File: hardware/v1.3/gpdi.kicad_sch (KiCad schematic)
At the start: 19 parts, among them J2 GPDI_C_1.3, U1 ECP5-CABGA256, U5 PCA9306DC1

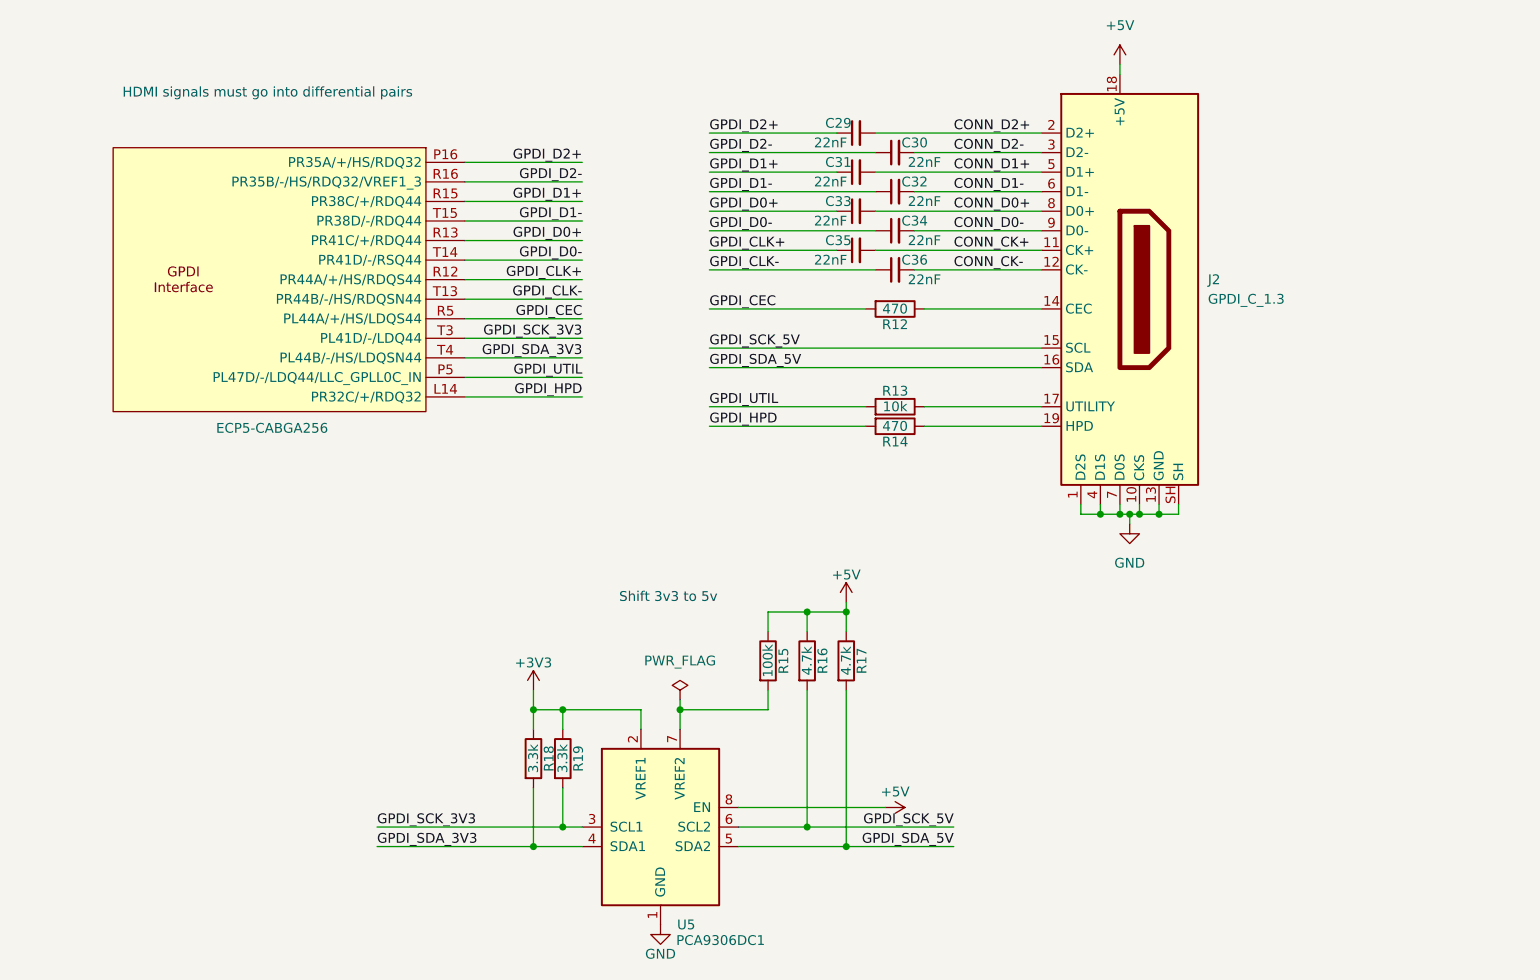
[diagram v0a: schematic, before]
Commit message: Update files
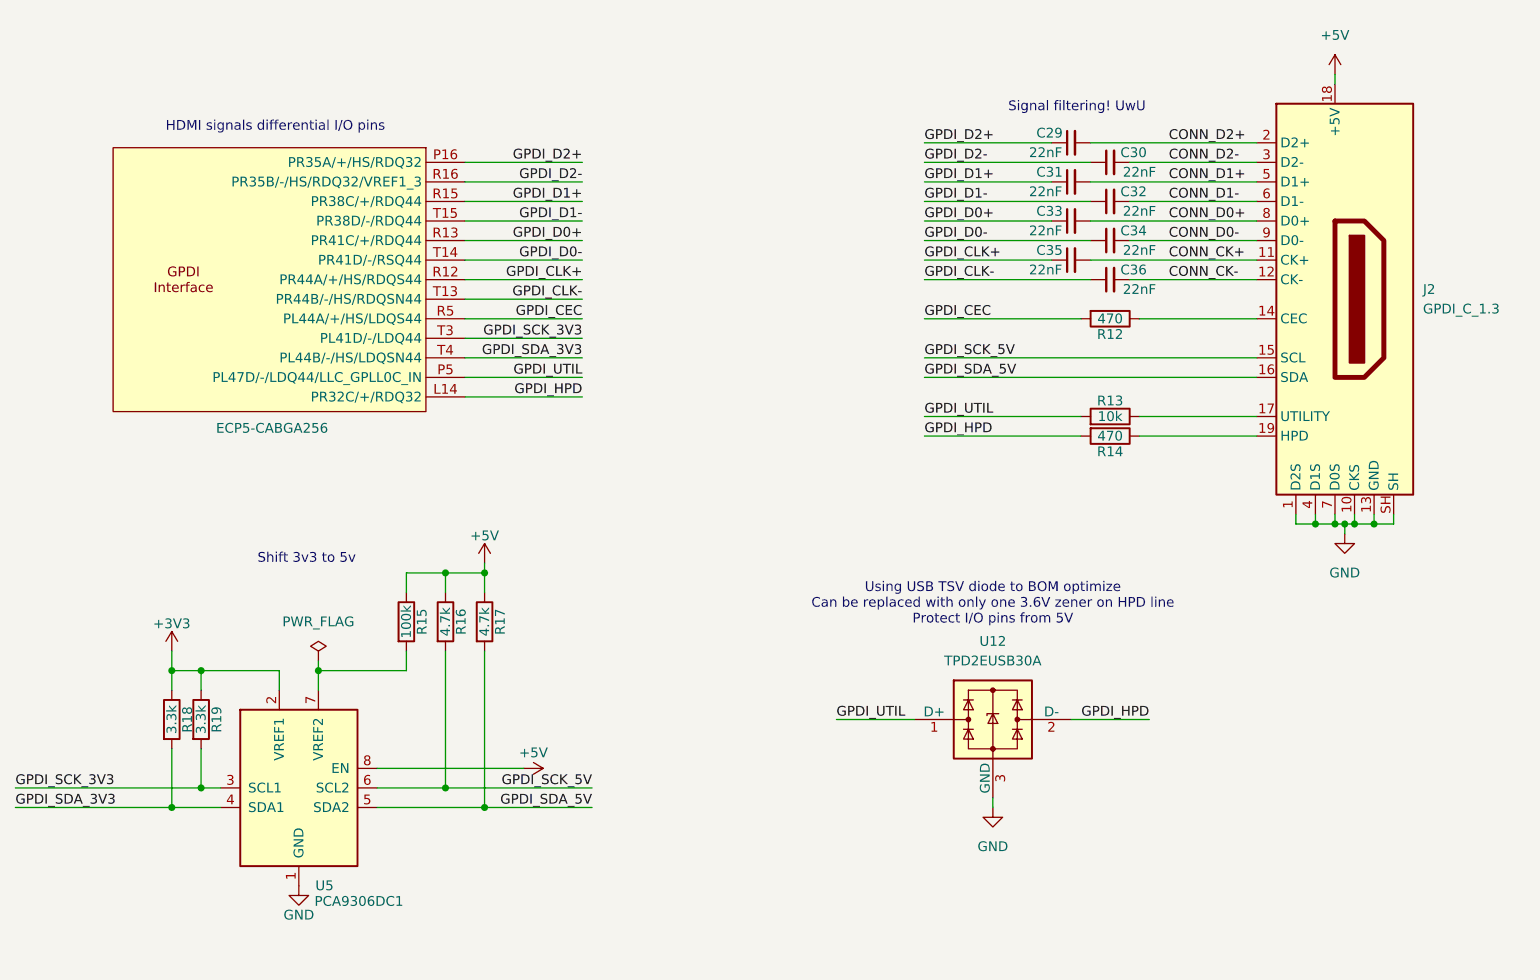
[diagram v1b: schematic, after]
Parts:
- added U12: TPD2EUSB30A, Package_TO_SOT_SMD:Texas_DRT-3, symbol Power_Protection:TPD2EUSB30A
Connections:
- net GND: now also U12.3 (GND)
- net GPDI_HPD: now also U12.2 (D-)
- net GPDI_UTIL: now also U12.1 (D+)
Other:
- note added: "HDMI signals differential I/O pins"
- note added: "Signal filtering! UwU"
- note added: "Using USB TSV diode to BOM optimize Can be replaced with only one 3.6V zener on HPD line Protect I/O pins from 5V"
- note removed: "HDMI signals must go into differential pairs"
- moved on the sheet: C29, C30, C31, C32, C33, C34, C35, C36, J2, R12, R13, R14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
